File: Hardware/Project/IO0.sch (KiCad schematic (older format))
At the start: 2 parts, among them U1 8255, U2 74LS138

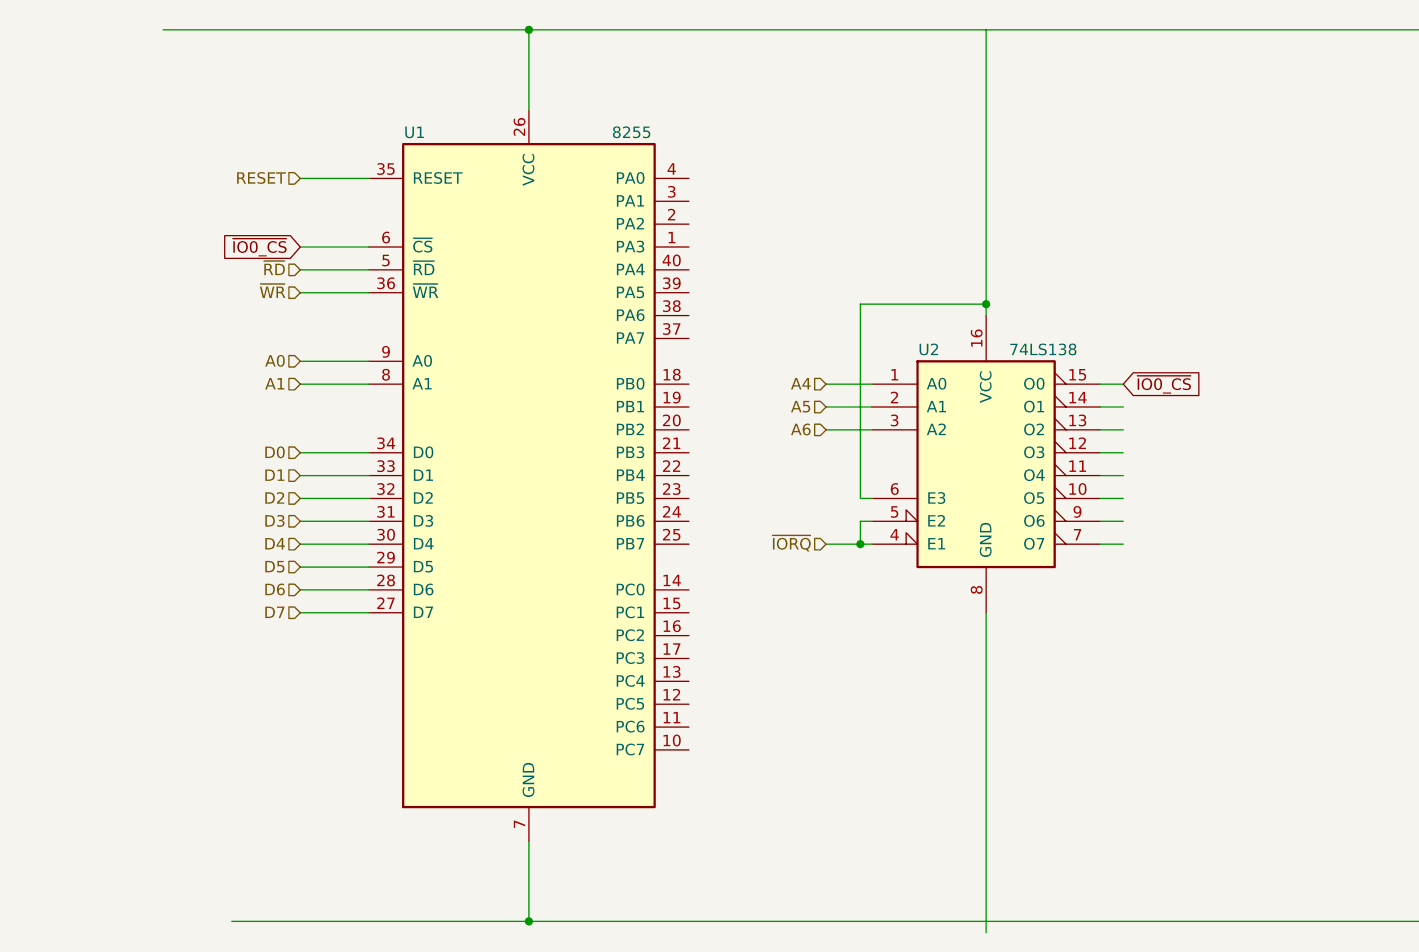
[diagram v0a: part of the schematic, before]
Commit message: 1
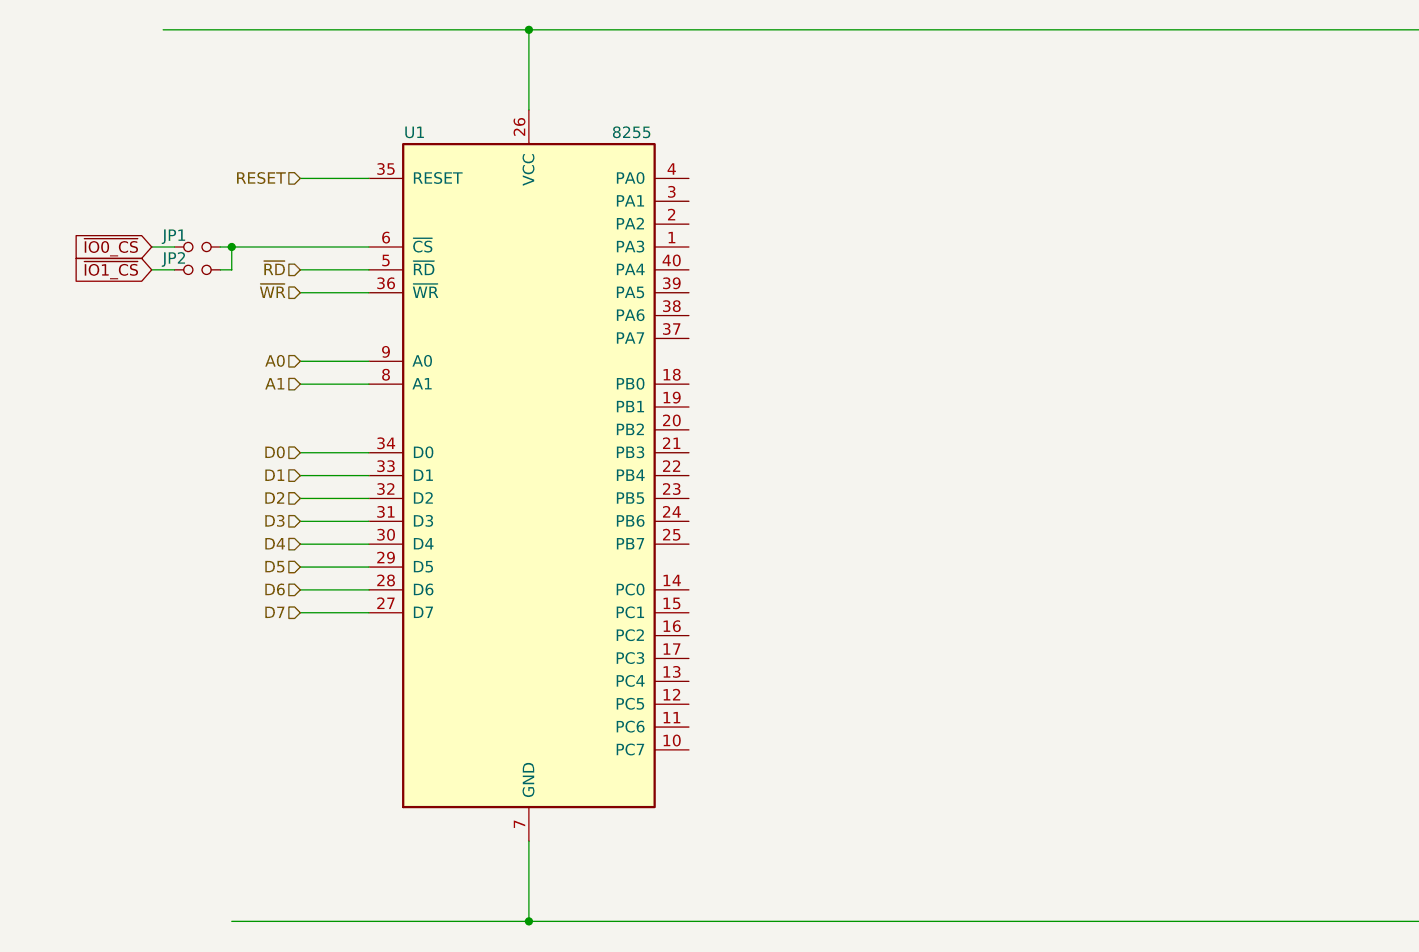
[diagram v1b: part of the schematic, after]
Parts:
- removed U2: 74LS138, Package_DIP:DIP-18_W7.62mm_Socket, symbol 74xx:74LS138
- added JP1, JP2: (no value), Jumper:SolderJumper-2_P1.3mm_Open_RoundedPad1.0x1.5mm, symbol Device:Jumper_NO_Small
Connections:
- net labels added: ~IO1_CS
- net labels removed: A4, A5, A6, ~IORQ
- wire segments 41 -> 25
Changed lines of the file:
@@
 $Descr A3 16535 11693
 encoding utf-8
-Sheet 2 6
+Sheet 2 5
 Title ""
 Date ""
@@
 	2050 2300 1750 2300
 Wire Wire Line
-	2050 2100 1750 2100
-Wire Wire Line
 	1150 1150 2750 1150
 Wire Wire Line
@@
 	2750 4700 2750 5050
 Connection ~ 2750 5050
-Wire Wire Line
-	2750 5050 15750 5050
 Text HLabel 1750 1800 0    50   Input ~ 0
 RESET
 Wire Wire Line
 	2050 1800 1750 1800
+Wire Wire Line
+	2750 5050 15750 5050
+Text GLabel 1100 2100 0    50   Input ~ 0
+~IO0_CS
+Text GLabel 1100 2200 0    50   Input ~ 0
+~IO1_CS
 $Comp
-L 74xx:74LS138 U?
-U 1 1 5D73DAC7
-P 4750 3000
-AR Path="/5C68B4BB/5D73DAC7" Ref="U?"  Part="1"
-AR Path="/5DED3C2A/5D73DAC7" Ref="U2"  Part="1"
-AR Path="/5D59EC5C/5D73DAC7" Ref="U?"  Part="1"
-AR Path="/5D62F4AC/5D73DAC7" Ref="U?"  Part="1"
-F 0 "U2" H 4500 3450 50  0000 C CNN
-F 1 "74LS138" H 5000 3450 50  0000 C CNN
-F 2 "Package_DIP:DIP-18_W7.62mm_Socket" H 4750 3000 50  0001 C CNN
-F 3 "http://www.ti.com/lit/gpn/sn74LS138" H 4750 3000 50  0001 C CNN
-	1    4750 3000
+L Device:Jumper_NO_Small JP1
+U 1 1 5DCA1D18
+P 1300 2100
+F 0 "JP1" H 1200 2150 50  0000 C CNN
+F 1 " " H 1300 2194 50  0000 C CNN
+F 2 "Jumper:SolderJumper-2_P1.3mm_Open_RoundedPad1.0x1.5mm" H 1300 2100 50  0001 C CNN
+F 3 "~" H 1300 2100 50  0001 C CNN
+	1    1300 2100
+	1    0    0    -1
+$EndComp
+$Comp
+L Device:Jumper_NO_Small JP2
+U 1 1 5DCA24B6
+P 1300 2200
+F 0 "JP2" H 1200 2250 50  0000 C CNN
+F 1 " " H 1300 2294 50  0000 C CNN
+F 2 "Jumper:SolderJumper-2_P1.3mm_Open_RoundedPad1.0x1.5mm" H 1300 2200 50  0001 C CNN
+F 3 "~" H 1300 2200 50  0001 C CNN
+	1    1300 2200
 	1    0    0    -1
 $EndComp
 Wire Wire Line
-	4750 2400 4750 2350
+	1200 2100 1100 2100
 Wire Wire Line
-	4750 3700 4750 5100
-Text HLabel 4050 2900 0    50   Input ~ 0
-A6
-Text HLabel 4050 2800 0    50   Input ~ 0
-A5
-Text HLabel 4050 2700 0    50   Input ~ 0
-A4
+	1200 2200 1100 2200
 Wire Wire Line
-	4250 2700 4050 2700
+	1400 2100 1450 2100
 Wire Wire Line
-	4250 2800 4050 2800
+	1450 2100 1450 2200
 Wire Wire Line
-	4250 2900 4050 2900
+	1400 2200 1450 2200
 Wire Wire Line
-	4250 3300 4200 3300
-Wire Wire Line
-	4200 3300 4200 3400
-Wire Wire Line
-	4200 3400 4250 3400
-Wire Wire Line
-	4250 3200 4200 3200
-Wire Wire Line
-	4200 3200 4200 2350
-Wire Wire Line
-	4200 2350 4750 2350
-Connection ~ 4750 2350
-Wire Wire Line
-	4750 2350 4750 1150
-Text GLabel 5350 2700 2    50   Input ~ 0
-~IO0_CS
-Connection ~ 4200 3400
-Wire Wire Line
-	5350 2700 5250 2700
-Text HLabel 4050 3400 0    50   Input ~ 0
-~IORQ
-Wire Wire Line
-	4050 3400 4200 3400
-Wire Wire Line
-	5350 2800 5250 2800
-Wire Wire Line
-	5350 2900 5250 2900
-Wire Wire Line
-	5350 3000 5250 3000
-Wire Wire Line
-	5350 3100 5250 3100
-Wire Wire Line
-	5350 3200 5250 3200
-Wire Wire Line
-	5350 3300 5250 3300
-Wire Wire Line
-	5350 3400 5250 3400
-Text GLabel 1750 2100 0    50   Input ~ 0
-~IO0_CS
+	1450 2100 2050 2100
+Connection ~ 1450 2100
 $EndSCHEMATC

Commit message: 1
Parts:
- added C5: 1uf, Capacitor_SMD:C_0805_2012Metric, symbol Device:C
- added J3: PSX_JOYPAD_1, Connector_PinSocket_2.54mm:PinSocket_1x09_P2.54mm_Vertical, symbol Connector:Conn_01x09_Female
- added J4: PSX_JOYPAD_2, Connector_PinSocket_2.54mm:PinSocket_1x09_P2.54mm_Vertical, symbol Connector:Conn_01x09_Female
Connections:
- net labels added: PSX_CLK, PSX_CMD, PSX_DAT, ~PSX_ACK, ~PSX_SEL_0, ~PSX_SEL_1
- wire segments 25 -> 58
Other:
- moved on the sheet: JP1, JP2, U1
